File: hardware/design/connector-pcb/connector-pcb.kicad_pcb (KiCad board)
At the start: 2 copper layers, 42 x 13 mm, 7 parts, among them J1 JWPF B04B, J2 JWPF B03B/B02B, J3 Conn_01x03_Pin, J5 Conn_01x02_Pin, J6 Conn_01x02_Pin, J8 JWPF B03B/B02B, J9 Conn_01x03_Pin

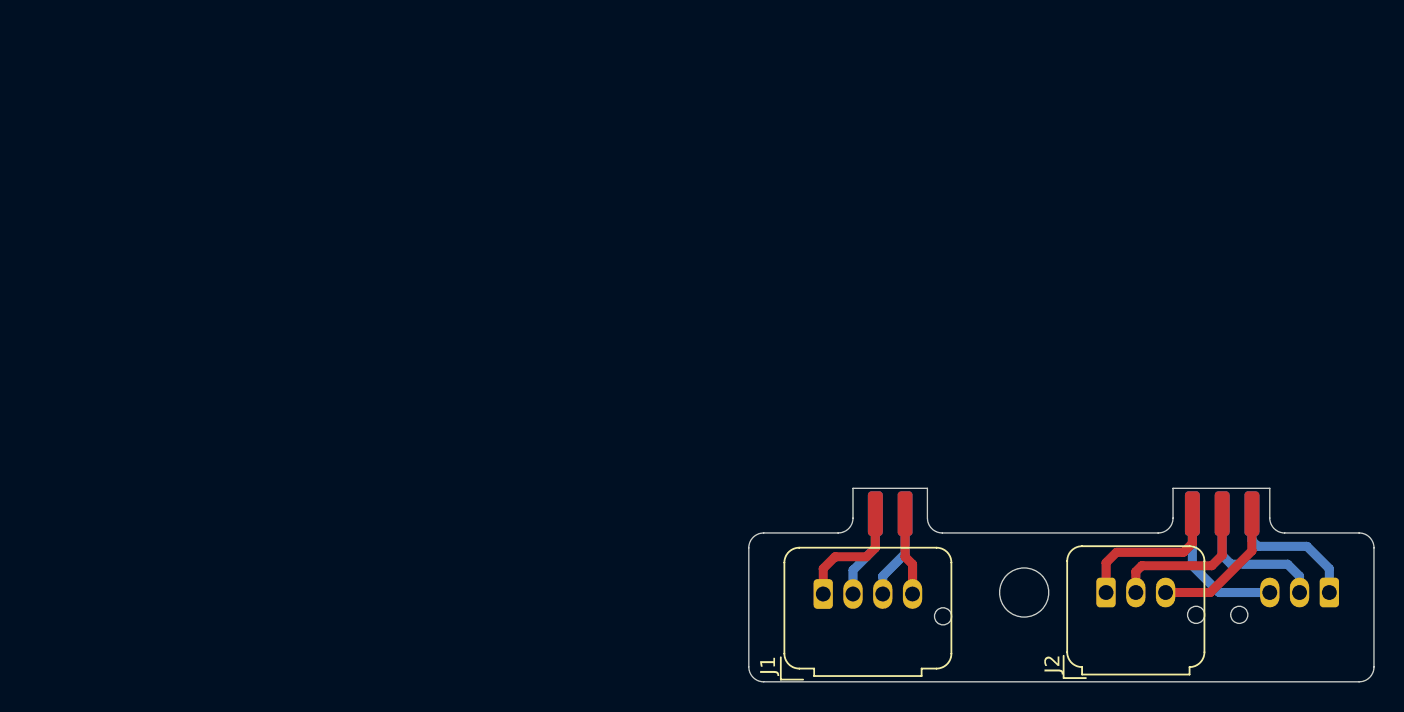
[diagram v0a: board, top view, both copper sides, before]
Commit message: Finalizing hardware design
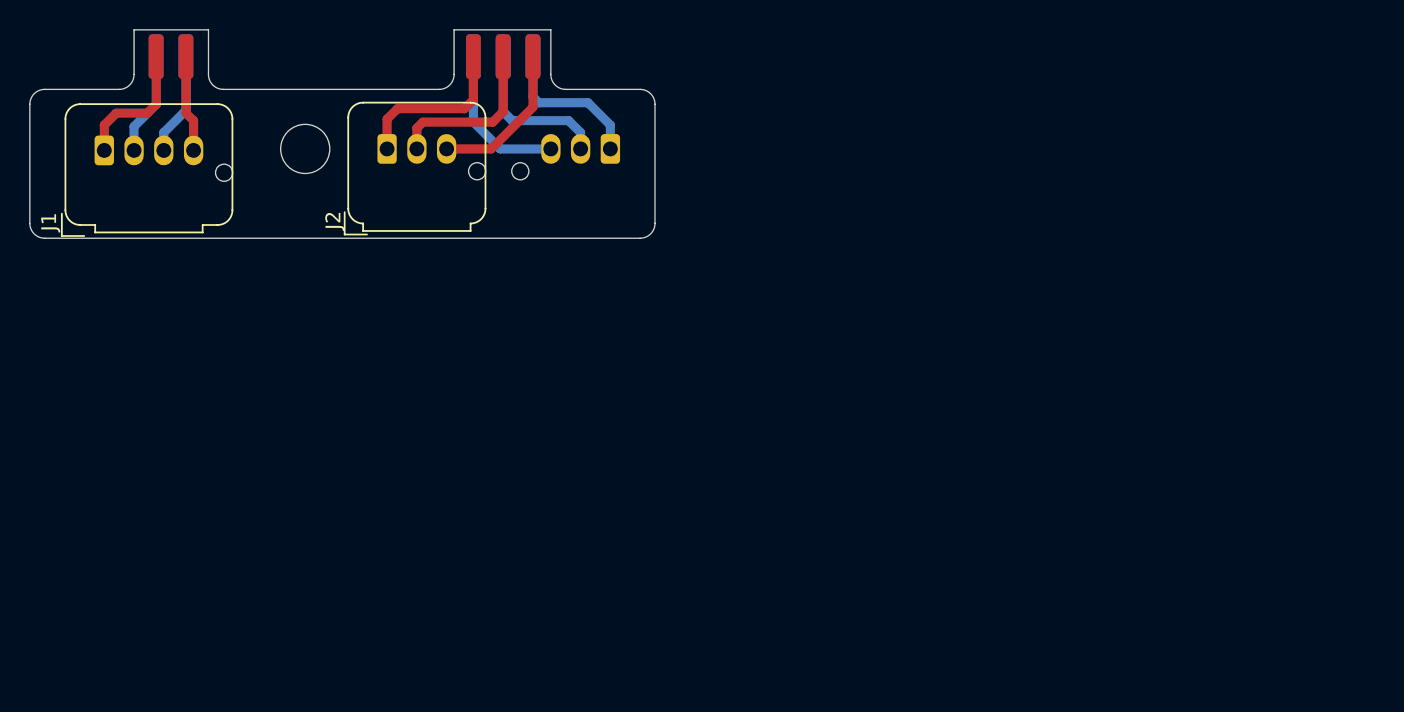
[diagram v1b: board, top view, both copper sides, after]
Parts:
- moved J5 57.2 mm to (92.7, 64.0)
- moved J6 57.2 mm to (92.7, 64.0)
- moved J3 57.2 mm to (115.0, 64.0)
- moved J9 57.2 mm to (115.0, 64.0)
- moved J1 56.8 mm to (88.2, 70.3)
- moved J2 56.8 mm to (107.2, 70.2)
- moved J8 56.8 mm to (122.2, 70.2)
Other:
- board size 42 x 13 mm -> 42 x 14 mm
